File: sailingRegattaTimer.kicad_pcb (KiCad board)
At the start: 2 copper layers, 58 x 68 mm, 29 parts, among them J1 Power, J1-Red-1M1 Conn_01x02_Socket, J2 Digital/PWM, J2-Yel-2M1 Conn_01x02_Socket, J3 Analog, J3-Grn-3M1 J3-Grn-3M, J4 Digital/PWM, J4-Blu-5M1 J4-Blu-5M1, J5-5v-LED1 Conn_01x02_Socket, J6-Reset1 J6-Reset, J7-Ext-Buz1 Conn_01x02_Socket, J8-Pololu-VReg1 Conn_01x04_Socket, J9-Relay1 Conn_01x03_Socket

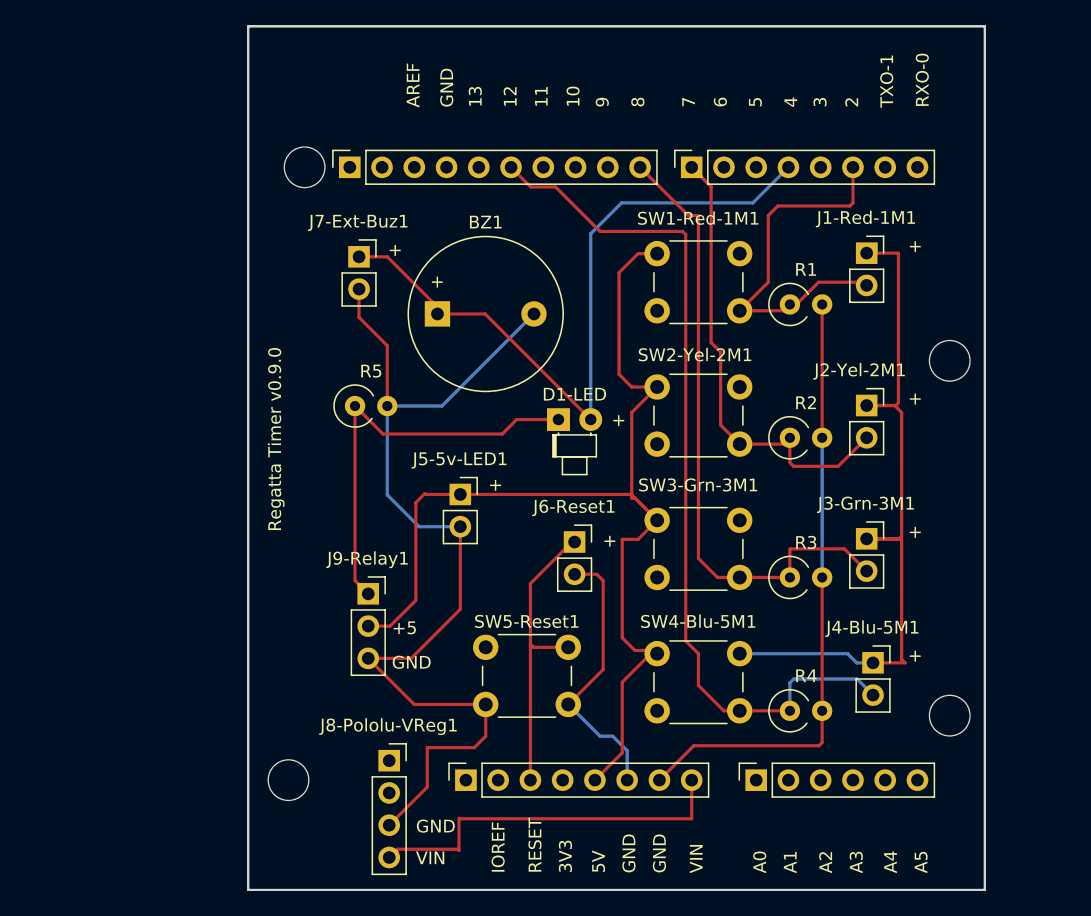
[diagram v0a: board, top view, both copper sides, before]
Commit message: save current working files
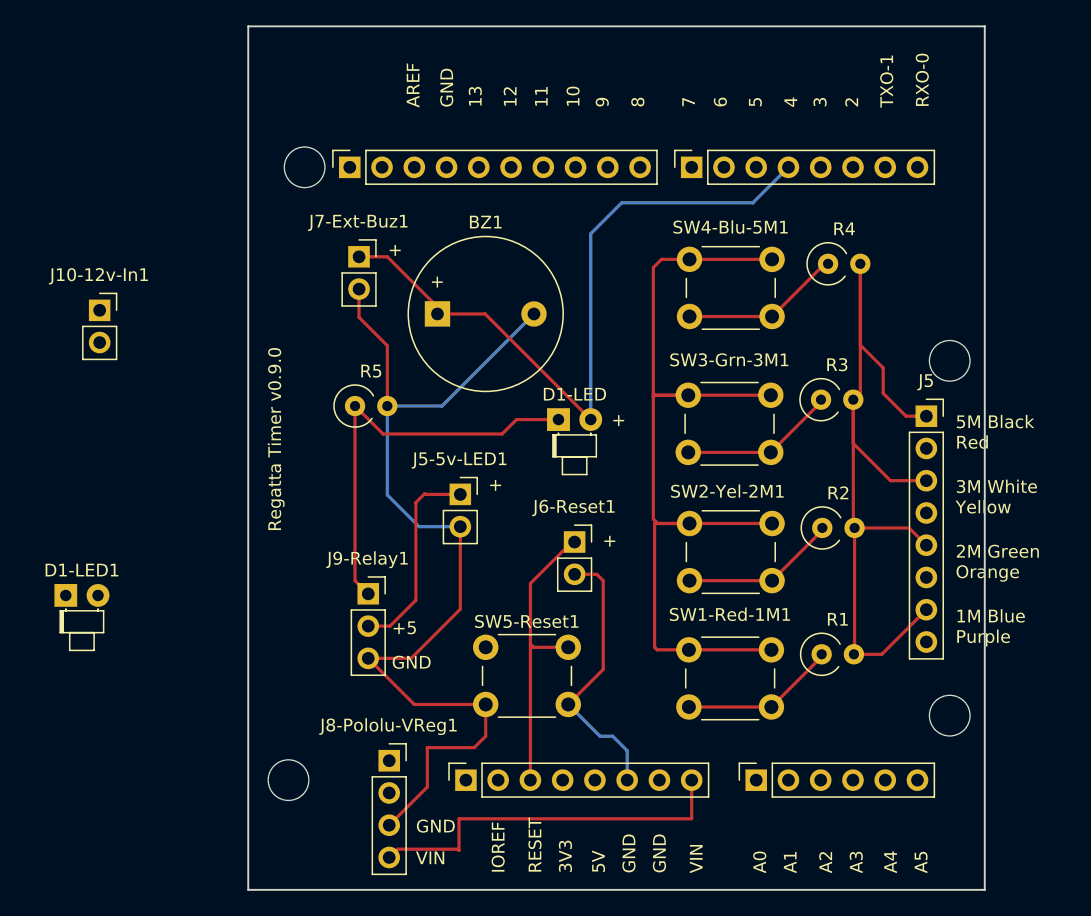
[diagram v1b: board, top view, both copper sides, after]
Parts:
- removed J1-Red-1M1, J2-Yel-2M1: Conn_01x02_Socket, Connector_PinSocket_2.54mm:PinSocket_1x02_P2.54mm_Vertical
- removed J3-Grn-3M1: J3-Grn-3M, Connector_PinSocket_2.54mm:PinSocket_1x02_P2.54mm_Vertical
- removed J4-Blu-5M1: J4-Blu-5M1, Connector_PinSocket_2.54mm:PinSocket_1x02_P2.54mm_Vertical
- added D1-LED1: LED, LED_THT:LED_D1.8mm_W1.8mm_H2.4mm_Horizontal_O1.27mm_Z1.6mm, F.Cu at (96.4, 82.9)
- added J10-12v-In1: Conn_01x02_Socket, Connector_PinSocket_2.54mm:PinSocket_1x02_P2.54mm_Vertical, F.Cu at (99.1, 60.5)
- added J5: Timers, Connector_PinSocket_2.54mm:PinSocket_1x08_P2.54mm_Vertical, F.Cu at (164.2, 68.8)
- moved R4 35.3 mm to (156.5, 56.8)
- moved SW1-Red-1M1 31.3 mm to (145.5, 87.2)
- moved SW4-Blu-5M1 31.2 mm to (145.6, 56.5)
- moved R1 27.7 mm to (156.0, 87.5)
- moved R3 14.2 mm to (155.9, 67.5)
- moved SW2-Yel-2M1 11.0 mm to (145.6, 77.2)
- moved SW3-Grn-3M1 10.2 mm to (145.4, 67.2)
- moved R2 7.54 mm to (156.0, 77.6)
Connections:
- BZ1 pad 1: /4 -> Net-(BZ1-+)
- BZ1 pad 2: GND -> Net-(BZ1--)
- J5-5v-LED1 pad 1: +5V -> Net-(J5-5v-LED1-Pin_1)
- J5-5v-LED1 pad 2: GND -> Net-(BZ1--)
- J6-Reset1 pad 1: /~{RESET} -> Net-(J6-Reset1-Pin_1)
- J6-Reset1 pad 2: GND -> Net-(BZ1--)
- J7-Ext-Buz1 pad 1: /4 -> Net-(BZ1-+)
- J7-Ext-Buz1 pad 2: GND -> Net-(BZ1--)
- J8-Pololu-VReg1 pad 2: unconnected-(J8-Pololu-VReg1-Pin_2-Pad2) -> Net-(J10-12v-In1-Pin_1)
- J8-Pololu-VReg1 pad 3: GND -> Net-(BZ1--)
- J8-Pololu-VReg1 pad 4: VCC -> Net-(J8-Pololu-VReg1-Pin_4)
- J9-Relay1 pad 1: Net-(D1-K) -> Net-(BZ1-+)
- J9-Relay1 pad 2: +5V -> Net-(J5-5v-LED1-Pin_1)
- J9-Relay1 pad 3: GND -> Net-(BZ1--)
- R1 pad 1: /2 -> Net-(J5-Pin_8)
- R1 pad 2: GND -> Net-(BZ1--)
- R2 pad 1: /7 -> Net-(J5-Pin_6)
- R2 pad 2: GND -> Net-(BZ1--)
- R3 pad 1: /8 -> Net-(J5-Pin_4)
- R3 pad 2: GND -> Net-(BZ1--)
- R4 pad 1: /12 -> Net-(J5-Pin_2)
- R4 pad 2: GND -> Net-(BZ1--)
- R5 pad 1: Net-(D1-K) -> Net-(D1-LED1-K)
- R5 pad 2: GND -> Net-(BZ1--)
- SW1-Red-1M1 pad 1: +5V -> Net-(J5-5v-LED1-Pin_1)
- SW1-Red-1M1 pad 2: /2 -> Net-(J5-Pin_8)
- SW2-Yel-2M1 pad 1: +5V -> Net-(J5-5v-LED1-Pin_1)
- SW2-Yel-2M1 pad 2: /7 -> Net-(J5-Pin_6)
- SW3-Grn-3M1 pad 1: +5V -> Net-(J5-5v-LED1-Pin_1)
- SW3-Grn-3M1 pad 2: /8 -> Net-(J5-Pin_4)
- SW4-Blu-5M1 pad 1: +5V -> Net-(J5-5v-LED1-Pin_1)
- SW4-Blu-5M1 pad 2: /12 -> Net-(J5-Pin_2)
- SW5-Reset1 pad 1: /~{RESET} -> Net-(J6-Reset1-Pin_1)
- SW5-Reset1 pad 2: GND -> Net-(BZ1--)
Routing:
- net Net-(BZ1--): track 0.00 -> 149.3 mm
- net +5V: track 145.0 -> 0.00 mm
- net GND: track 149.2 -> 21.8 mm
- net Net-(J5-5v-LED1-Pin_1): track 0.00 -> 89.0 mm
- net /12: track 69.3 -> 0.00 mm
- net /8: track 50.0 -> 0.00 mm
- net /7: track 36.4 -> 0.00 mm
- net /2: track 29.3 -> 0.00 mm
- net Net-(J5-Pin_2): track 0.00 -> 12.6 mm
- net Net-(J5-Pin_8): track 0.00 -> 12.3 mm
- net Net-(J5-Pin_4): track 0.00 -> 12.3 mm
- net Net-(J5-Pin_6): track 0.00 -> 12.3 mm
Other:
- board text added: "1M Blue Purple"
- board text added: "2M Green Orange"
- board text added: "3M White Yellow"
- board text added: "5M Black Red"
